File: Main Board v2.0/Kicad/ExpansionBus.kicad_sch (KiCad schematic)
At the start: 1 part, among them J1 Bus_ISA_16bit

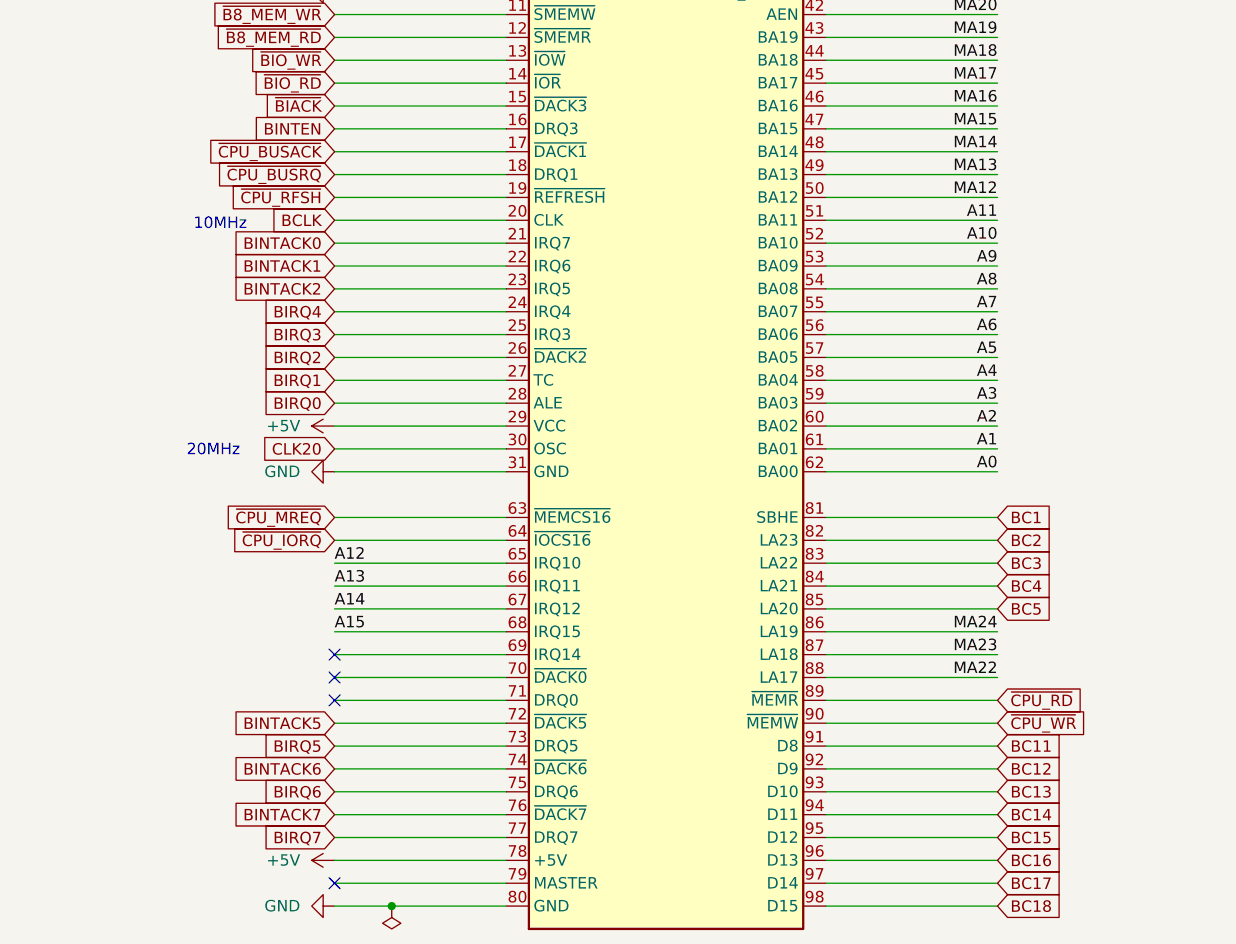
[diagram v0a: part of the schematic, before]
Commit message: board rev a routed
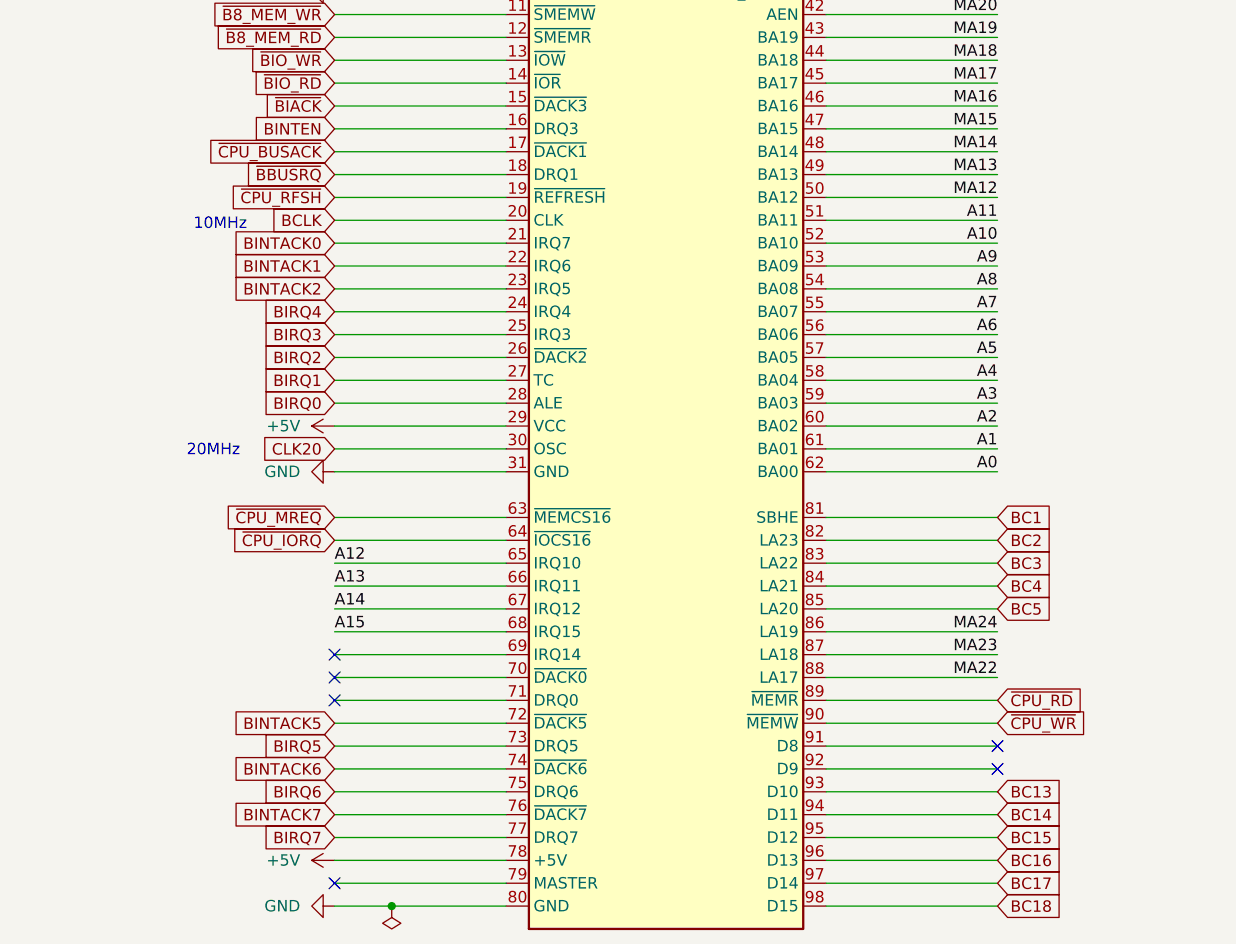
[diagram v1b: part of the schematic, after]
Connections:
- net BC11: no longer names the net of J1.91 (D8)
- net BC12: no longer names the net of J1.92 (D9)
- net ~{CPU_BUSRQ} renamed ~{BBUSRQ}
- no-connect marks 4 -> 6
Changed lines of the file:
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@@
 	)
 	(no_connect
+		(at 160.02 135.89)
+	)
+	(no_connect
+		(at 160.02 133.35)
+	)
+	(no_connect
 		(at 86.36 123.19)
 	)
@@
 		)
 	)
-	(global_label "~{CPU_BUSRQ}"
+	(global_label "~{BBUSRQ}"
 		(shape input)
 		(at 86.36 69.85 180)
@@
 		)
 		(property "Intersheetrefs" "${INTERSHEET_REFS}"
-			(at 72.1262 69.85 0)
+			(at 75.6943 69.85 0)
 			(hide yes)
 			(show_name no)
@@
 		)
 	)
-	(global_label "BC12"
-		(shape input)
-		(at 160.02 135.89 0)
-		(fields_autoplaced yes)
-		(effects
-			(font
-				(size 1.27 1.27)
-			)
-			(justify left)
-		)
-		(property "Intersheetrefs" "${INTERSHEET_REFS}"
-			(at 167.9642 135.89 0)
-			(hide yes)
-			(show_name no)
-			(do_not_autoplace no)
-			(effects
-				(font
-					(size 1.27 1.27)
-				)
-				(justify left)
-			)
-		)
-	)
 	(global_label "BIRQ4"
 		(shape input)
@@
 			)
 		)
-	)
-	(global_label "BC11"
-		(shape input)
-		(at 160.02 133.35 0)
-		(fields_autoplaced yes)
-		(effects
-			(font
-				(size 1.27 1.27)
-			)
-			(justify left)
-		)
-		(property "Intersheetrefs" "${INTERSHEET_REFS}"
-			(at 167.9642 133.35 0)
-			(hide yes)
-			(show_name no)
-			(do_not_autoplace no)
-			(effects
-				(font
-					(size 1.27 1.27)
-				)
-				(justify left)
-			)
-		)
